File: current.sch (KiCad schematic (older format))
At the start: 42 parts, among them Q401 CJ2302, Q402 CJ2302, Q403 CJ2302, Q404 CJ2302, U401 MAX9919FASA+, U402 MAX9919FASA+, U403 MAX9919FASA+, U404 MAX9919FASA+, U405 MAX9919FASA+

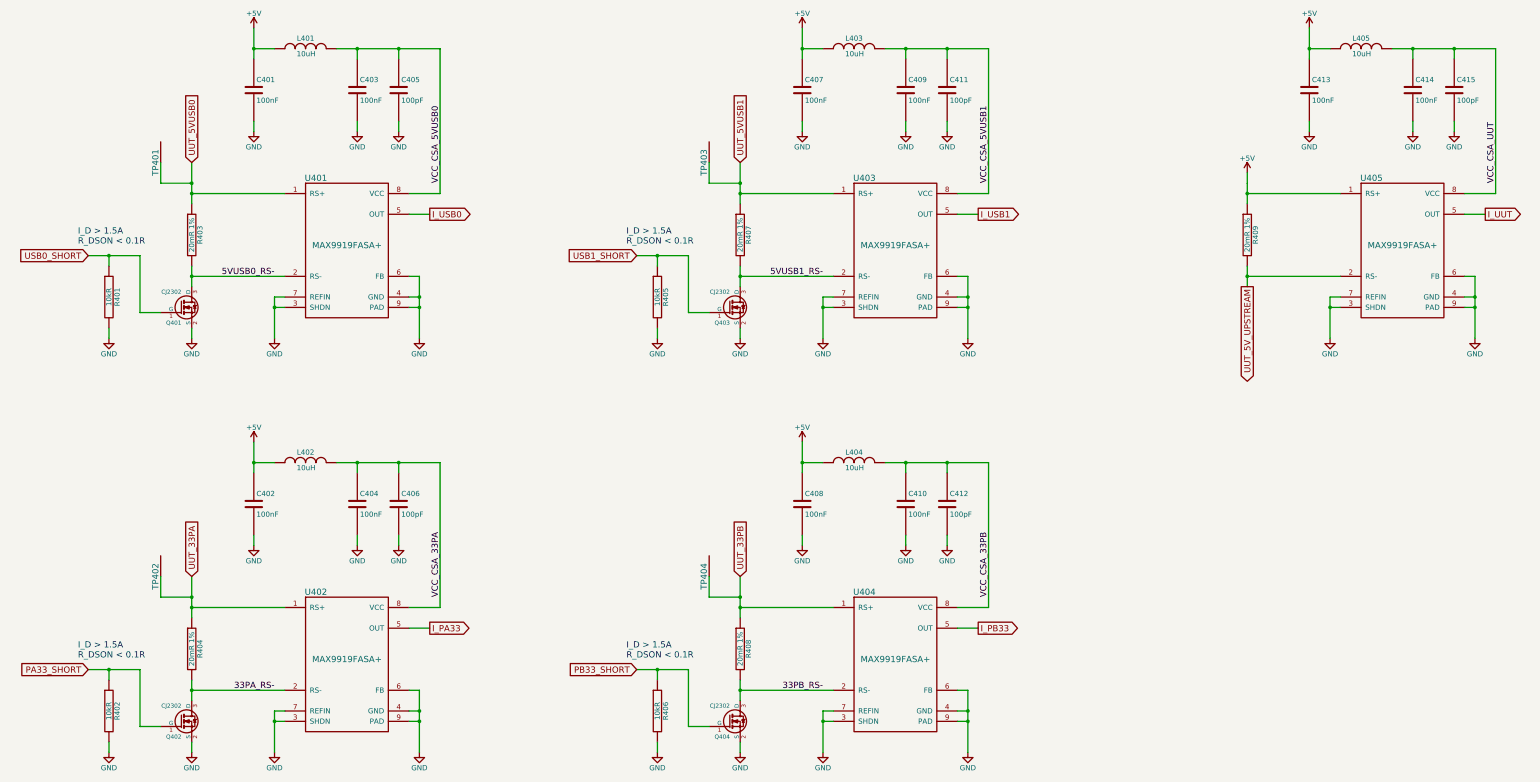
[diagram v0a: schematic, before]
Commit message: annotated, netlist
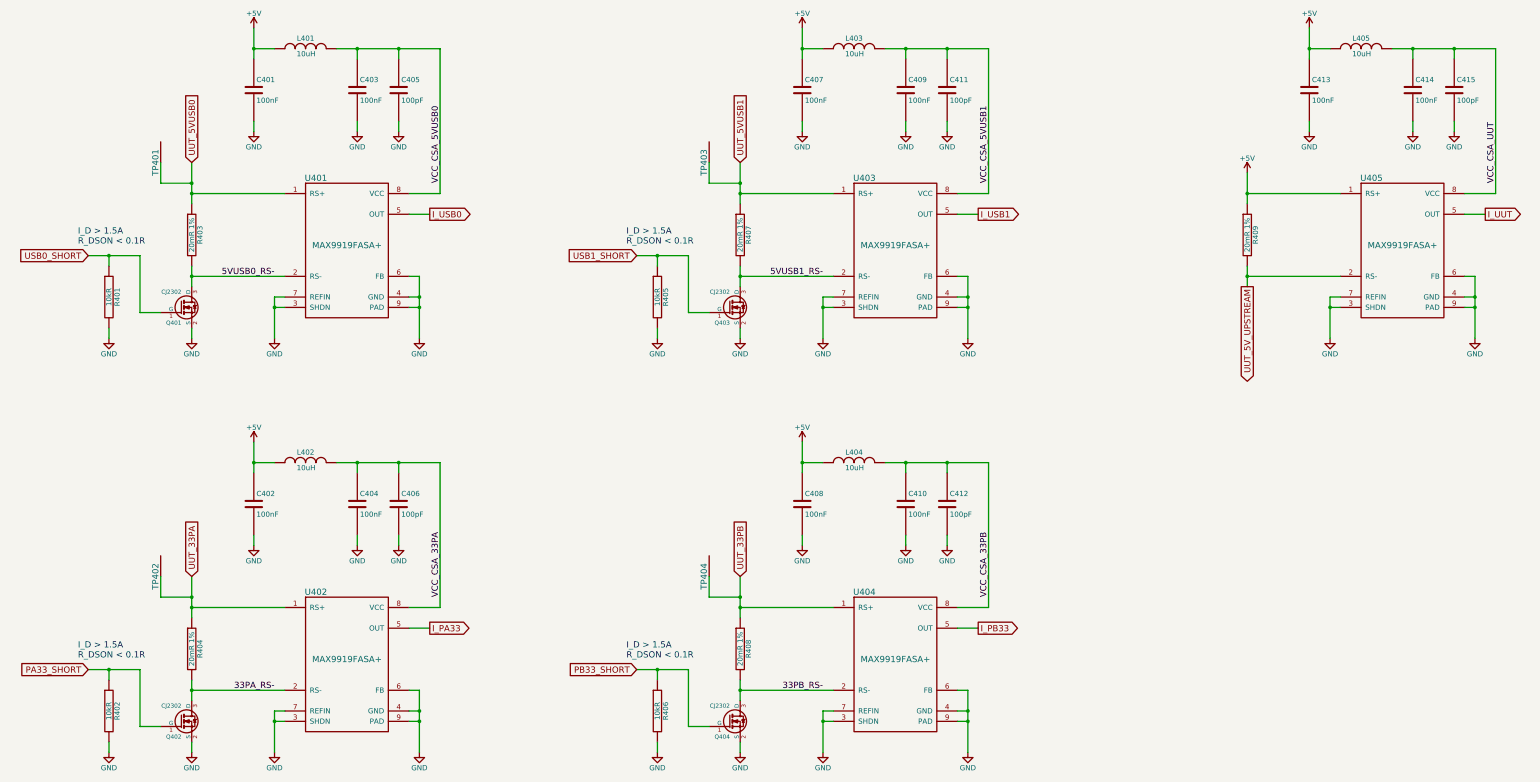
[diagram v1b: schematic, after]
